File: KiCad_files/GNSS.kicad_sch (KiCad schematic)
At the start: 1 part

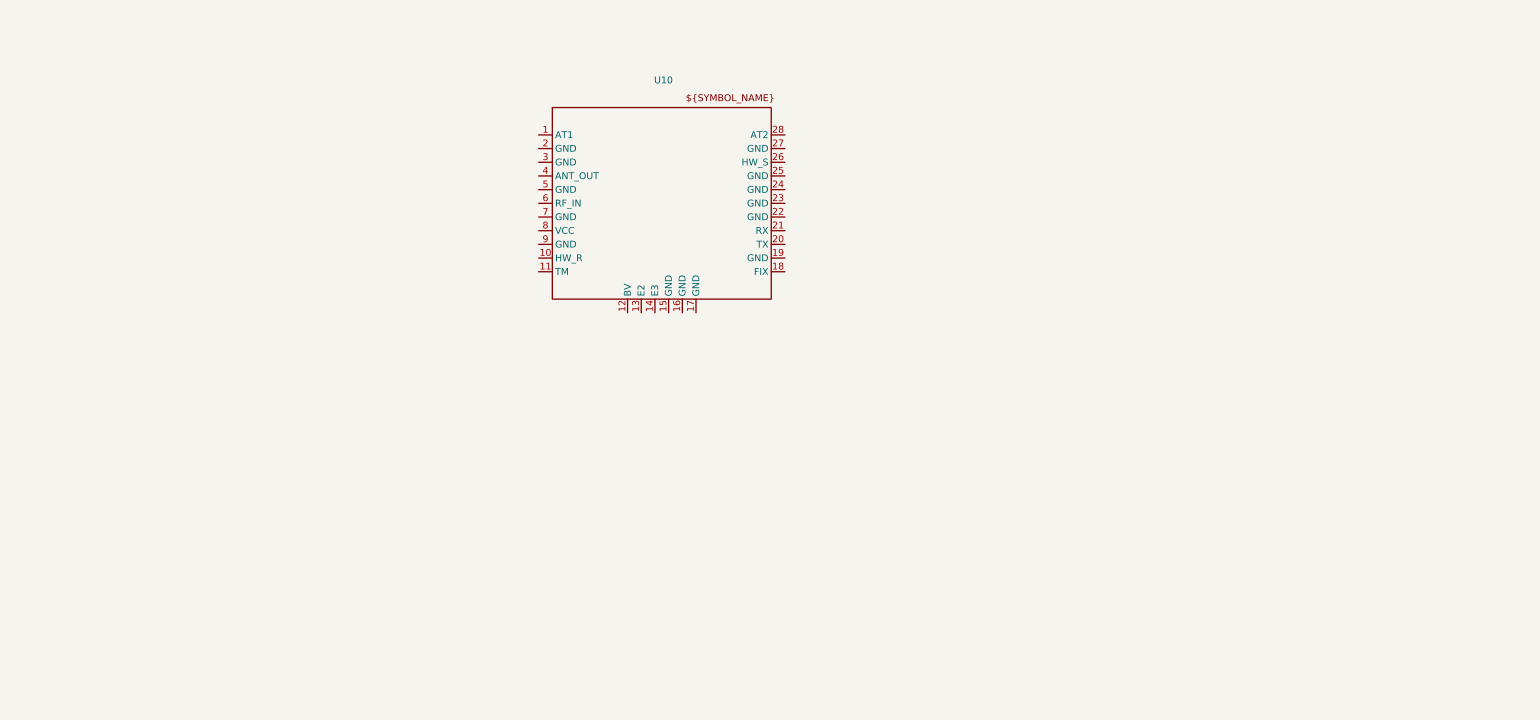
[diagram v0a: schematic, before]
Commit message: GNSS aloitettu
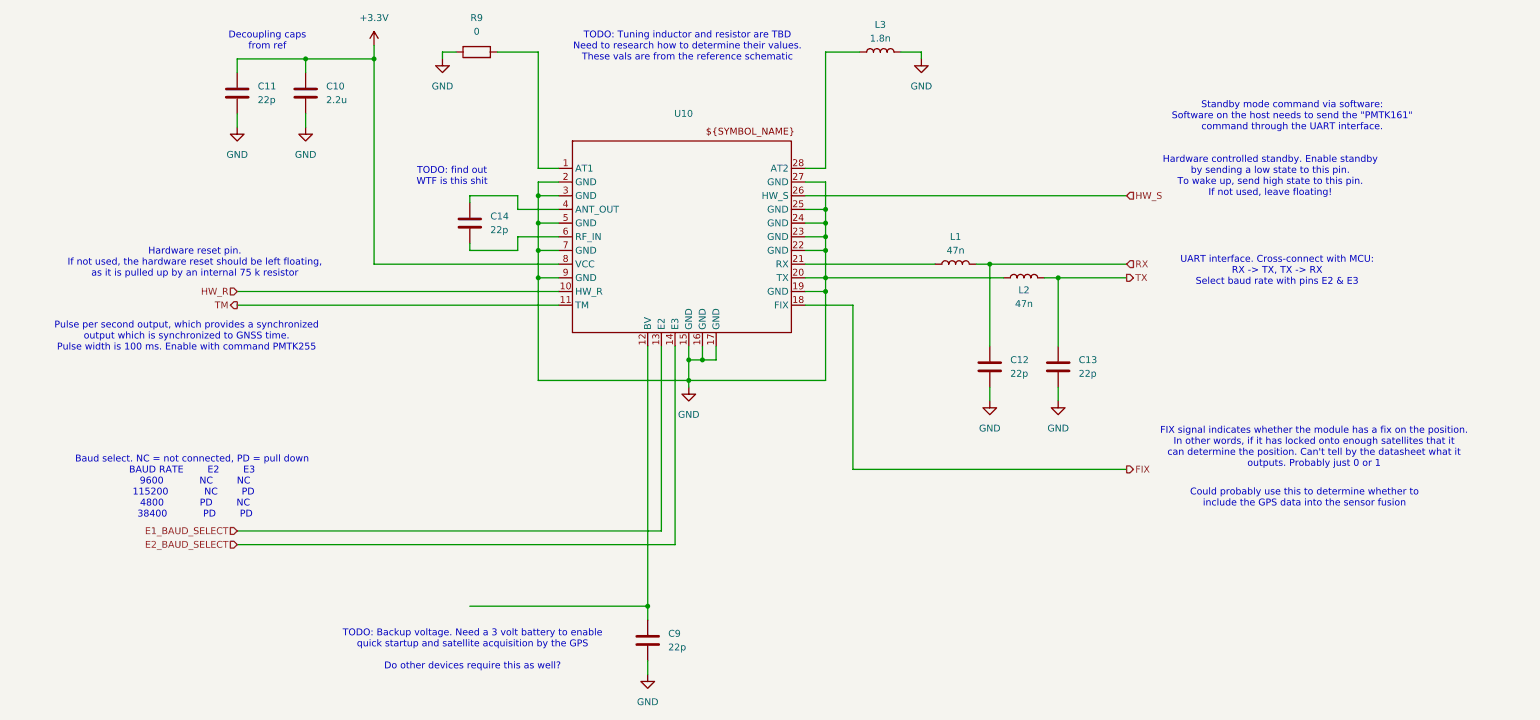
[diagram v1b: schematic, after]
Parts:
- added C10: 2.2u, symbol Device:C
- added C11, C12, C13, C14, C9: 22p, symbol Device:C
- added L1, L2: 47n, symbol Device:L
- added L3: 1.8n, symbol Device:L
- added R9: 0, symbol Device:R
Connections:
- net at U10.1 (AT1): now also R9.2
- net HW_R: now reaches U10.10 (HW_R)
- net TM: now reaches U10.11 (TM)
- net at U10.12 (BV): now also C9.1
- net E1_BAUD_SELECT: now reaches U10.13 (E2)
- net E2_BAUD_SELECT: now reaches U10.14 (E3)
- net GND: now reaches U10.15 (GND)
- net GND: now also U10.16 (GND), U10.17 (GND), U10.19 (GND), U10.2 (GND), U10.20 (TX), U10.22 (GND), U10.23 (GND), U10.24 (GND), U10.25 (GND), U10.27 (GND), U10.3 (GND), U10.5 (GND), U10.7 (GND), U10.9 (GND), C10.2, C11.2, C12.2, C13.2, C9.2, L2.1, L3.2, R9.1
- net FIX: now reaches U10.18 (FIX)
- net at U10.21 (RX): now also L1.1
- net HW_S: now reaches U10.26 (HW_S)
- net at U10.28 (AT2): now also L3.1
- net at U10.4 (ANT_OUT): now also C14.1
- net at U10.6 (RF_IN): now also C14.2
- net +3.3V: now reaches U10.8 (VCC)
- net +3.3V: now also C10.1, C11.1
- new net RX: C12.1, L1.2
- new net TX: C13.1, L2.2
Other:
- note added: "Baud select. NC = not connected, PD = pull down BAUD RATE E2 E3 9600 NC NC 115200 NC PD 4800 PD NC 38400 PD PD"
- note added: "Could probably use this to determine whether to include the GPS data into the sensor fusion"
- note added: "Decoupling caps from ref"
- note added: "FIX signal indicates whether the module has a fix on the position. In other words, if it has locked onto enough satellites that it can determine the position. Can't tell by the datasheet what it outputs. Probably just 0 or 1"
- note added: "Hardware controlled standby. Enable standby by sending a low state to this pin. To wake up, send high state to this pin. If not used, leave floating!"
- note added: "Hardware reset pin. If not used, the hardware reset should be left floating, as it is pulled up by an internal 75 k resistor"
- note added: "Pulse per second output, which provides a synchronized output which is synchronized to GNSS time. Pulse width is 100 ms. Enable with command PMTK255"
- note added: "Standby mode command via software: Software on the host needs to send the "PMTK161" command through the UART interface."
- note added: "TODO: Backup voltage. Need a 3 volt battery to enable quick startup and satellite acquisition by the GPS Do other devices require this as well?"
- note added: "TODO: Tuning inductor and resistor are TBD Need to research how to determine their values. These vals are from the reference schematic"
- note added: "TODO: find out WTF is this shit"
- note added: "UART interface. Cross-connect with MCU: RX -> TX, TX -> RX Select baud rate with pins E2 & E3"
